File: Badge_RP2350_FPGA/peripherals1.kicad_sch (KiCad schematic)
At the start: 21 parts, among them J3 Conn_01x15_Pin, J4 Conn_01x15_Pin

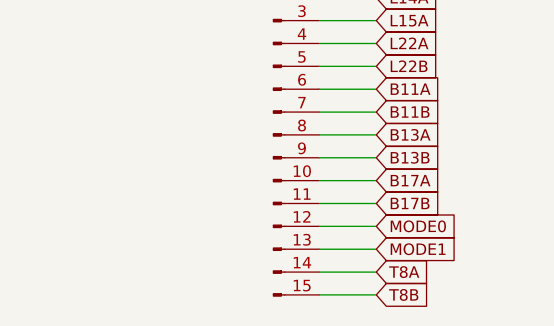
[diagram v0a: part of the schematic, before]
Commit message: put pull up to mode1, pull down to mode0
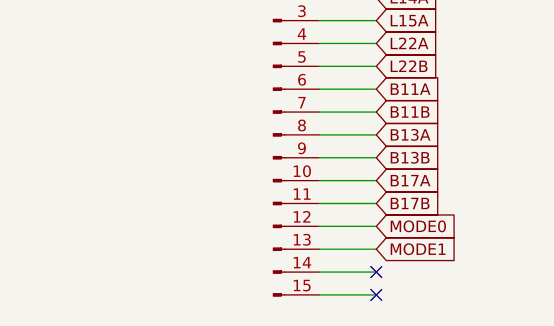
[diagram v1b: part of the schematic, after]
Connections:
- net T8A: no longer names the net of J4.14 (Pin_14)
- net T8B: no longer names the net of J4.15 (Pin_15)
- no-connect marks 0 -> 2
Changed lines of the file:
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@@
 		(color 0 0 0 0)
 	)
+	(no_connect
+		(at 177.8 119.38)
+	)
+	(no_connect
+		(at 177.8 121.92)
+	)
 	(wire
 		(pts
@@
 		)
 	)
-	(global_label "T8B"
-		(shape input)
-		(at 177.8 121.92 0)
-		(fields_autoplaced yes)
-		(effects
-			(font
-				(size 1.27 1.27)
-			)
-			(justify left)
-		)
-		(property "Intersheetrefs" "${INTERSHEET_REFS}"
-			(at 184.2323 121.92 0)
-			(hide yes)
-			(show_name no)
-			(do_not_autoplace no)
-			(effects
-				(font
-					(size 1.27 1.27)
-				)
-				(justify left)
-			)
-		)
-	)
 	(global_label "B11B"
 		(shape input)
@@
 			(hide yes)
 			(show_name no)
-			(do_not_autoplace no)
-			(effects
-				(font
-					(size 1.27 1.27)
-				)
-				(justify left)
-			)
-		)
-	)
-	(global_label "T8A"
-		(shape input)
-		(at 177.8 119.38 0)
-		(fields_autoplaced yes)
-		(effects
-			(font
-				(size 1.27 1.27)
-			)
-			(justify left)
-		)
-		(property "Intersheetrefs" "${INTERSHEET_REFS}"
-			(at 184.0509 119.38 0)
-			(hide yes)
-			(show_name no)
